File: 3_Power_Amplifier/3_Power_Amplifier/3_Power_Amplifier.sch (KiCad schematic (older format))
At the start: 24 parts, among them P1 SIGNAL_INPUT_SMA, P10 SWITCHED_POWER_INV, P11 SIGNAL_INPUT, P12 SWITCHED_POWER_INV, P2 SWITCHED_POWER_INV, P3 ISLETA, P4 ISLETA, P5 ISLETA, P6 ISLETA, P7 SIGNAL_INPUT, P8 TIERRA, P9 TIERRA, Q1 IRF740NPBF, Q2 IRF740NPBF, Q3 IRF740NPBF, Q4 IRF740NPBF

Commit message: GENERADOR_V8
ORGANIZACION DE ELEMENTOS
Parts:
- R1, R2, R3, R4, R5, R6, R7, R8: footprint libreria_Power_Amplifier_huellas:INV_R_0805_HandSoldering -> Resistors_SMD:R_0805_HandSoldering
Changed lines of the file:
@@
 	3200 6400 650  6400
-$Comp
-L 100 R1
-U 1 1 59D2EF68
-P 3750 2500
-F 0 "R1" H 3780 2520 50  0000 L CNN
-F 1 "100" H 3780 2460 50  0000 L CNN
-F 2 "libreria_Power_Amplifier_huellas:INV_R_0805_HandSoldering" H 3680 2420 50  0001 C CNN
-F 3 "" H 3750 2500 50  0000 C CNN
-	1    3750 2500
-	0    1    1    0
-$EndComp
-$Comp
-L 100 R3
-U 1 1 59D2F0DF
-P 5650 2450
-F 0 "R3" H 5680 2470 50  0000 L CNN
-F 1 "100" H 5680 2410 50  0000 L CNN
-F 2 "libreria_Power_Amplifier_huellas:INV_R_0805_HandSoldering" H 5580 2370 50  0001 C CNN
-F 3 "" H 5650 2450 50  0000 C CNN
-	1    5650 2450
-	0    1    1    0
-$EndComp
-$Comp
-L 100 R5
-U 1 1 59D2F33F
-P 7450 2400
-F 0 "R5" H 7480 2420 50  0000 L CNN
-F 1 "100" H 7480 2360 50  0000 L CNN
-F 2 "libreria_Power_Amplifier_huellas:INV_R_0805_HandSoldering" H 7380 2320 50  0001 C CNN
-F 3 "" H 7450 2400 50  0000 C CNN
-	1    7450 2400
-	0    1    1    0
-$EndComp
-$Comp
-L 100 R7
-U 1 1 59D2F4DC
-P 9200 2400
-F 0 "R7" H 9230 2420 50  0000 L CNN
-F 1 "100" H 9230 2360 50  0000 L CNN
-F 2 "libreria_Power_Amplifier_huellas:INV_R_0805_HandSoldering" H 9130 2320 50  0001 C CNN
-F 3 "" H 9200 2400 50  0000 C CNN
-	1    9200 2400
-	0    1    1    0
-$EndComp
-$Comp
-L 10K R2
-U 1 1 59D2FB7B
-P 4000 2700
-F 0 "R2" H 4030 2720 50  0000 L CNN
-F 1 "10K" H 4030 2660 50  0000 L CNN
-F 2 "libreria_Power_Amplifier_huellas:INV_R_0805_HandSoldering" H 3930 2620 50  0001 C CNN
-F 3 "" H 4000 2700 50  0000 C CNN
-	1    4000 2700
-	1    0    0    -1
-$EndComp
-$Comp
-L 10K R4
-U 1 1 59D2FC1D
-P 5900 2650
-F 0 "R4" H 5930 2670 50  0000 L CNN
-F 1 "10K" H 5930 2610 50  0000 L CNN
-F 2 "libreria_Power_Amplifier_huellas:INV_R_0805_HandSoldering" H 5830 2570 50  0001 C CNN
-F 3 "" H 5900 2650 50  0000 C CNN
-	1    5900 2650
-	1    0    0    -1
-$EndComp
-$Comp
-L 10K R6
-U 1 1 59D2FFBD
-P 7600 2650
-F 0 "R6" H 7630 2670 50  0000 L CNN
-F 1 "10K" H 7630 2610 50  0000 L CNN
-F 2 "libreria_Power_Amplifier_huellas:INV_R_0805_HandSoldering" H 7530 2570 50  0001 C CNN
-F 3 "" H 7600 2650 50  0000 C CNN
-	1    7600 2650
-	1    0    0    -1
-$EndComp
-$Comp
-L 10K R8
-U 1 1 59D301F0
-P 9400 2650
-F 0 "R8" H 9430 2670 50  0000 L CNN
-F 1 "10K" H 9430 2610 50  0000 L CNN
-F 2 "libreria_Power_Amplifier_huellas:INV_R_0805_HandSoldering" H 9330 2570 50  0001 C CNN
-F 3 "" H 9400 2650 50  0000 C CNN
-	1    9400 2650
-	1    0    0    -1
-$EndComp
 $Comp
 L SIGNAL_INPUT_SMA P1
@@
 	-1   0    0    1
 $EndComp
+$Comp
+L 100 R1
+U 1 1 59DA5392
+P 3750 2500
+F 0 "R1" H 3780 2520 50  0000 L CNN
+F 1 "100" H 3780 2460 50  0000 L CNN
+F 2 "Resistors_SMD:R_0805_HandSoldering" H 3680 2420 50  0001 C CNN
+F 3 "" H 3750 2500 50  0000 C CNN
+	1    3750 2500
+	0    1    1    0
+$EndComp
+$Comp
+L 100 R7
+U 1 1 59DA55F1
+P 9200 2400
+F 0 "R7" H 9230 2420 50  0000 L CNN
+F 1 "100" H 9230 2360 50  0000 L CNN
+F 2 "Resistors_SMD:R_0805_HandSoldering" H 9130 2320 50  0001 C CNN
+F 3 "" H 9200 2400 50  0000 C CNN
+	1    9200 2400
+	0    1    1    0
+$EndComp
+$Comp
+L 100 R3
+U 1 1 59DA62D7
+P 5650 2450
+F 0 "R3" H 5680 2470 50  0000 L CNN
+F 1 "100" H 5680 2410 50  0000 L CNN
+F 2 "Resistors_SMD:R_0805_HandSoldering" H 5580 2370 50  0001 C CNN
+F 3 "" H 5650 2450 50  0000 C CNN
+	1    5650 2450
+	0    1    1    0
+$EndComp
+$Comp
+L 100 R5
+U 1 1 59DA63EB
+P 7450 2400
+F 0 "R5" H 7480 2420 50  0000 L CNN
+F 1 "100" H 7480 2360 50  0000 L CNN
+F 2 "Resistors_SMD:R_0805_HandSoldering" H 7380 2320 50  0001 C CNN
+F 3 "" H 7450 2400 50  0000 C CNN
+	1    7450 2400
+	0    1    1    0
+$EndComp
+$Comp
+L 10K R2
+U 1 1 59DA72F3
+P 4000 2700
+F 0 "R2" H 4030 2720 50  0000 L CNN
+F 1 "10K" H 4030 2660 50  0000 L CNN
+F 2 "Resistors_SMD:R_0805_HandSoldering" H 3930 2620 50  0001 C CNN
+F 3 "" H 4000 2700 50  0000 C CNN
+	1    4000 2700
+	1    0    0    -1
+$EndComp
+$Comp
+L 10K R4
+U 1 1 59DA76ED
+P 5900 2650
+F 0 "R4" H 5930 2670 50  0000 L CNN
+F 1 "10K" H 5930 2610 50  0000 L CNN
+F 2 "Resistors_SMD:R_0805_HandSoldering" H 5830 2570 50  0001 C CNN
+F 3 "" H 5900 2650 50  0000 C CNN
+	1    5900 2650
+	1    0    0    -1
+$EndComp
+$Comp
+L 10K R6
+U 1 1 59DA7B59
+P 7600 2650
+F 0 "R6" H 7630 2670 50  0000 L CNN
+F 1 "10K" H 7630 2610 50  0000 L CNN
+F 2 "Resistors_SMD:R_0805_HandSoldering" H 7530 2570 50  0001 C CNN
+F 3 "" H 7600 2650 50  0000 C CNN
+	1    7600 2650
+	1    0    0    -1
+$EndComp
+$Comp
+L 10K R8
+U 1 1 59DA811D
+P 9400 2650
+F 0 "R8" H 9430 2670 50  0000 L CNN
+F 1 "10K" H 9430 2610 50  0000 L CNN
+F 2 "Resistors_SMD:R_0805_HandSoldering" H 9330 2570 50  0001 C CNN
+F 3 "" H 9400 2650 50  0000 C CNN
+	1    9400 2650
+	1    0    0    -1
+$EndComp
 $EndSCHEMATC

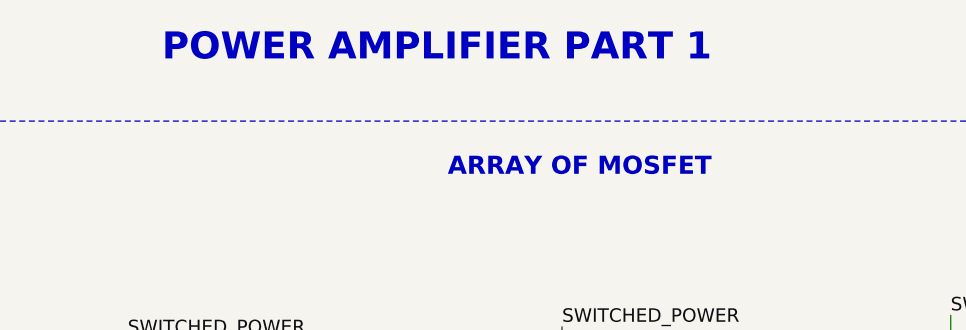
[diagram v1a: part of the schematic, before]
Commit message: GENERADOR V_14
ULTIMO DISEÑO CON LOGOS
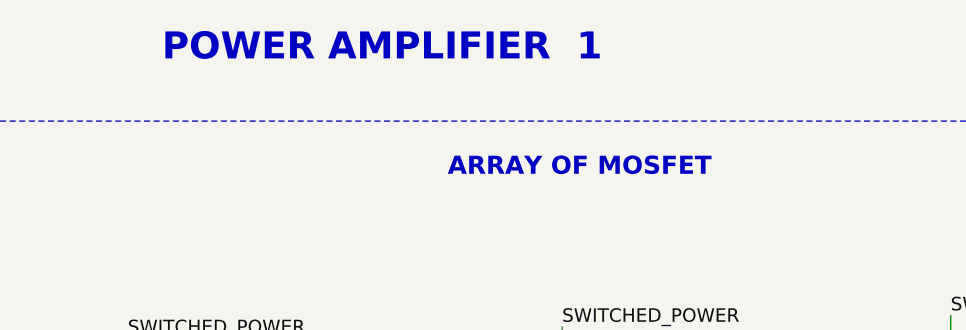
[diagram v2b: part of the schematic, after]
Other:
- note added: "POWER AMPLIFIER 1"
- note removed: "POWER AMPLIFIER PART 1"
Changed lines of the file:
@@
 	650  1150 650  6400
 Text Notes 4550 900  0    118  ~ 24
-POWER AMPLIFIER PART 1
+POWER AMPLIFIER  1
 Wire Wire Line
 	1100 3400 1900 3400
